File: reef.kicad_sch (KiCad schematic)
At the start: 63 parts, among them J1 nice!view sockets, J2 battery connector, SW0 B3U-1000P[], SW1 PCM12SMTR, U1 nice_nano, U2 TRRS, U3 TRRS

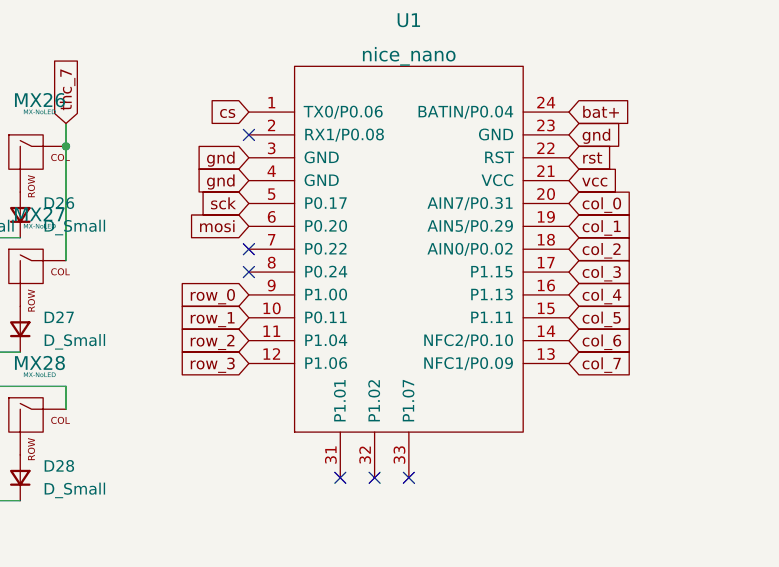
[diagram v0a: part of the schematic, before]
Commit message: Traces Routed
all traces should now be fully routed
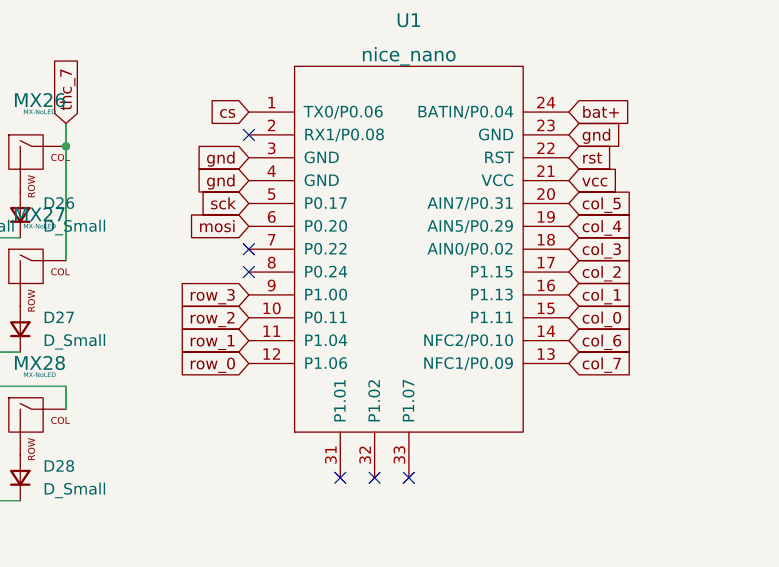
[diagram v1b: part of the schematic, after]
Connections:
- net col_0: now also U1.15 (P1.11); no longer U1.20 (AIN7/P0.31)
- net col_1: now also U1.16 (P1.13); no longer U1.19 (AIN5/P0.29)
- net col_2: now also U1.17 (P1.15); no longer U1.18 (AIN0/P0.02)
- net col_3: now also U1.18 (AIN0/P0.02); no longer U1.17 (P1.15)
- net col_4: now also U1.19 (AIN5/P0.29); no longer U1.16 (P1.13)
- net col_5: now also U1.20 (AIN7/P0.31); no longer U1.15 (P1.11)
- net row_0: now also U1.12 (P1.06); no longer U1.9 (P1.00)
- net row_1: now also U1.11 (P1.04); no longer U1.10 (P0.11)
- net row_2: now also U1.10 (P0.11); no longer U1.11 (P1.04)
- net row_3: now also U1.9 (P1.00); no longer U1.12 (P1.06)
